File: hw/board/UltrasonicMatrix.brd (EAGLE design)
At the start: 140 x 150 mm, 180 parts, among them IC1 7812L, U1 TC4427EOA, U10 TC4427EOA, U11 TC4427EOA, U12 TC4427EOA, U13 TC4427EOA, U14 TC4427EOA, U15 TC4427EOA, U16 TC4427EOA, U17 TC4427EOA, U18 TC4427EOA, U19 TC4427EOA, U2 TC4427EOA, U20 TC4427EOA, U21 TC4427EOA, U22 TC4427EOA, U23 TC4427EOA, U24 TC4427EOA, U25 TC4427EOA, U26 TC4427EOA, U27 TC4427EOA, U28 TC4427EOA, U29 TC4427EOA, U3 TC4427EOA, U30 TC4427EOA, U31 TC4427EOA, U32 TC4427EOA, U4 TC4427EOA, U5 TC4427EOA, U6 TC4427EOA, U7 TC4427EOA, U8 TC4427EOA, U9 TC4427EOA

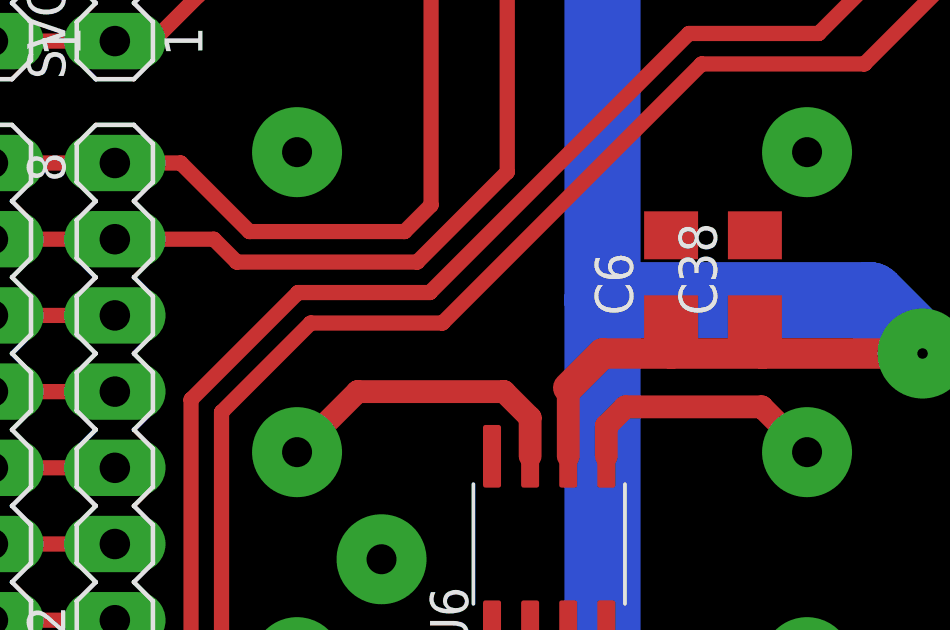
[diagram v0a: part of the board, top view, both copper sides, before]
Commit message: Board completed
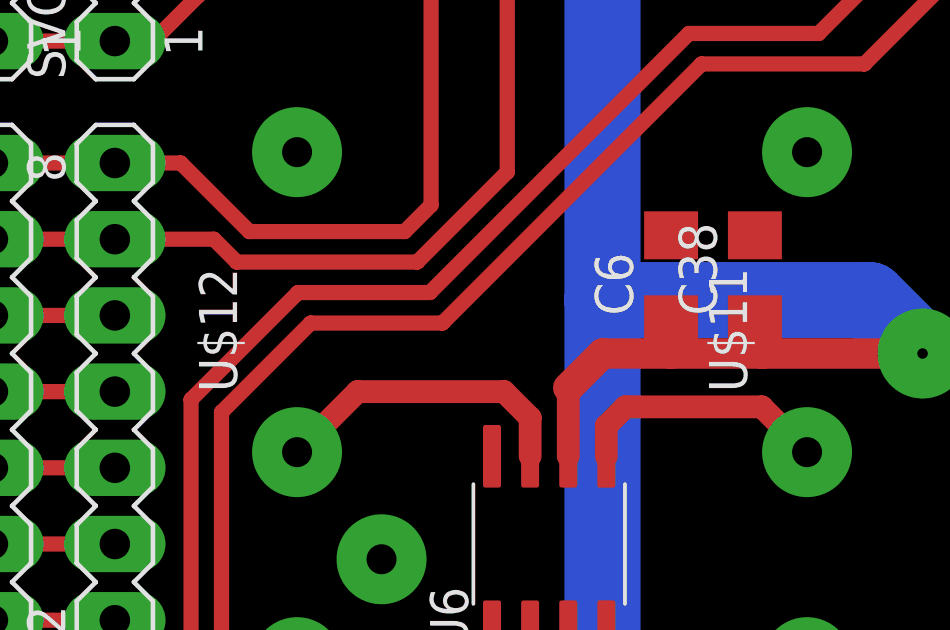
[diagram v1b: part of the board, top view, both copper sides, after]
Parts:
- U$8: device ultrasonic:TCT40-16 -> TCT40:TCT40-16
- flipped U$11 to the top
- flipped U$12 to the top
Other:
- board text added: "(1,1)"
- board text added: "(1,2)"
- board text added: "(1,3)"
- board text added: "(1,4)"
- board text added: "(1,5)"
- board text added: "(1,6)"
- board text added: "(1,7)"
- board text added: "(1,8)"
- board text added: "(2,1)"
- board text added: "(2,2)"
- board text added: "(2,3)"
- board text added: "(2,4)"
- board text added: "(2,5)"
- board text added: "(2,6)"
- board text added: "(2,7)"
- board text added: "(2,8)"
- board text added: "(3,1)"
- board text added: "(3,2)"
- board text added: "(3,3)"
- board text added: "(3,4)"
- board text added: "(3,5)"
- board text added: "(3,6)"
- board text added: "(3,7)"
- board text added: "(3,8)"
- board text added: "(4,1)"
- board text added: "(4,2)"
- board text added: "(4,3)"
- board text added: "(4,4)"
- board text added: "(4,5)"
- board text added: "(4,6)"
- board text added: "(4,7)"
- board text added: "(4,8)"
- board text added: "(5,1)"
- board text added: "(5,2)"
- board text added: "(5,3)"
- board text added: "(5,4)"
- board text added: "(5,5)"
- board text added: "(5,6)"
- board text added: "(5,7)"
- board text added: "(5,8)"
- board text added: "(6,1)"
- board text added: "(6,2)"
- board text added: "(6,3)"
- board text added: "(6,4)"
- board text added: "(6,5)"
- board text added: "(6,6)"
- board text added: "(6,7)"
- board text added: "(6,8)"
- board text added: "(7,1)"
- board text added: "(7,2)"
- board text added: "(7,3)"
- board text added: "(7,4)"
- board text added: "(7,5)"
- board text added: "(7,6)"
- board text added: "(7,7)"
- board text added: "(7,8)"
- board text added: "(8,1)"
- board text added: "(8,2)"
- board text added: "(8,3)"
- board text added: "(8,4)"
- board text added: "(8,5)"
- board text added: "(8,6)"
- board text added: "(8,7)"
- board text added: "(8,8)"
- board text added: "06"
- board text added: "07"
- board text added: "08"
- board text added: "09"
- board text added: "19VDC"
- board text added: "22"
- board text added: "24"
- board text added: "26"
- board text added: "28"
- board text added: "30"
- board text added: "32"
- board text added: "34"
- board text added: "36"
- board text added: "38"
- board text added: "40"
- board text added: "42"
- board text added: "44"
- board text added: "46"
- board text added: "48"
- board text added: "50"
- board text added: "52"
- board text removed: "18VDC"
